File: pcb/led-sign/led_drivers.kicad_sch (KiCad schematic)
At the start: 16 parts, among them U6 LP5024, U7 LP5024, U8 LP5024, U9 LP5024

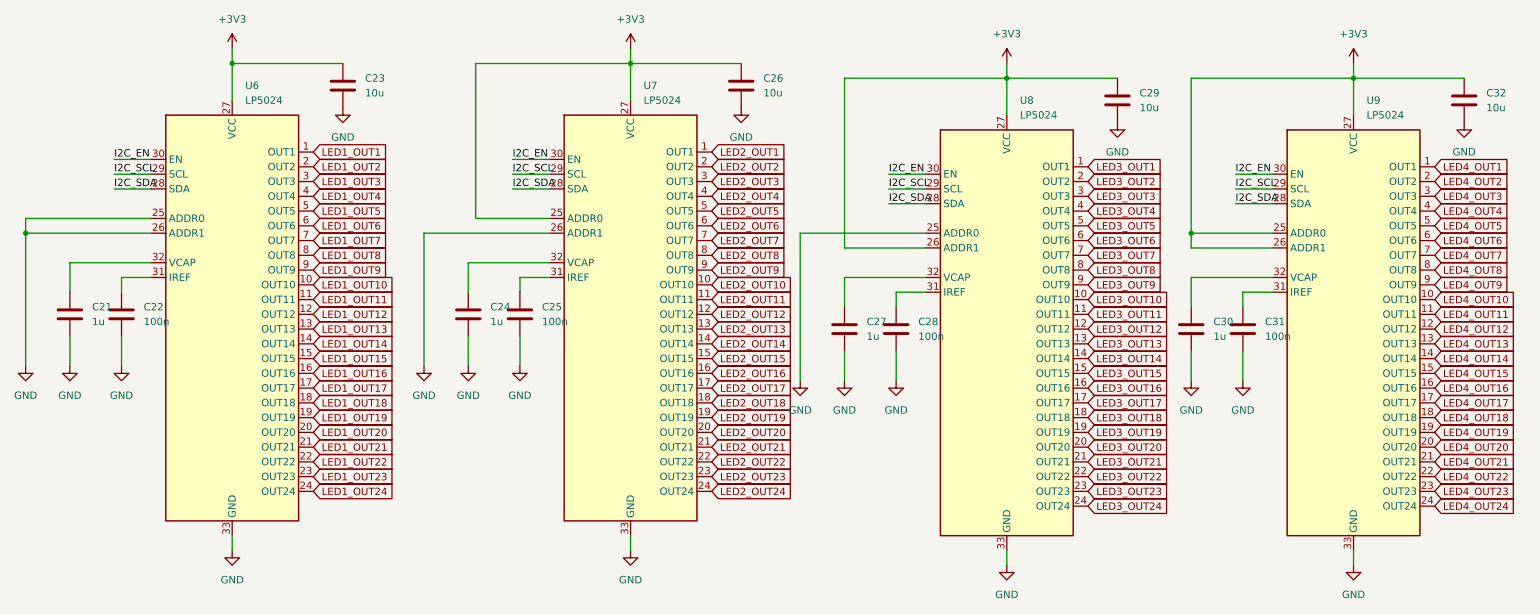
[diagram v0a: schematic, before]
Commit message: start layout
Signed-off-by: 3nt3 <gott@3nt3.de>
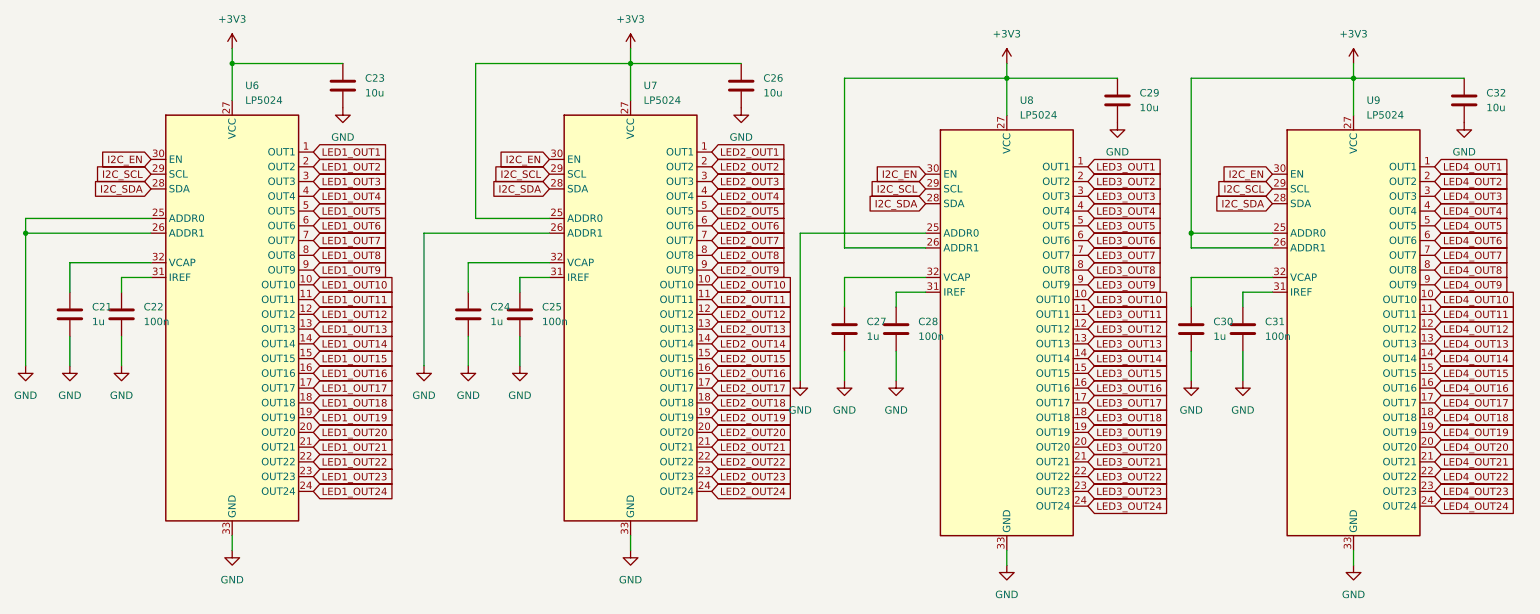
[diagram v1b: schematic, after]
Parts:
- C21, C22, C23, C24, C25, C26, C27, C28, C29, C30, C31, C32: footprint (none) -> Capacitor_SMD:C_0603_1608Metric_Pad1.08x0.95mm_HandSolder
- U6, U7, U8, U9: footprint (none) -> 3nt3:LP5024
